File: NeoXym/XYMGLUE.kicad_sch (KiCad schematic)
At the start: 42 parts, among them J1 Conn_01x08, J2 Conn_01x08, SW1 SW_Push, SW2 SW_Push, SW3 SW_SPDT, SW4 SW_SPDT, SW5 SW_Push, U1 74HCT138, U10 74HCT04, U15 74HCT00, U16 74HCT14, U17 74HCT121, U18 NE555P, U2 74HCT138, U4 74HCT32, U5 74HCT00, U6 74HCT09, U8 74HCT10, U9 74HCT00, X1 1.8432MHz

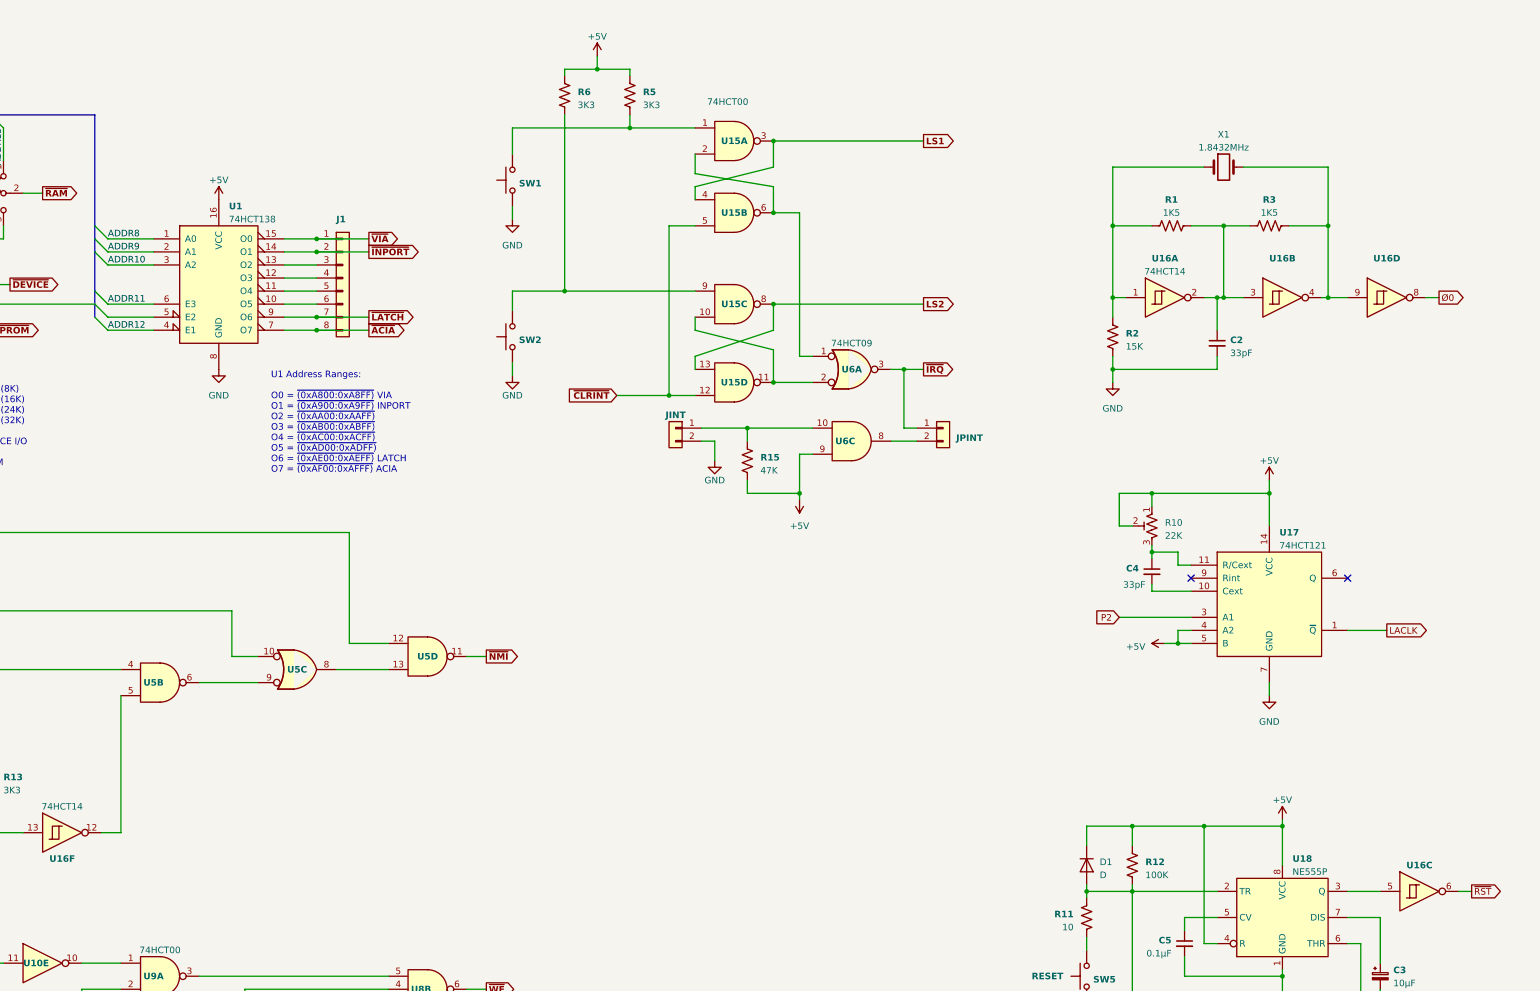
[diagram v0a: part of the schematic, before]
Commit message: modified:   CPU_MEM_IOCTRL.kicad_sch 	modified:   XYMGLUE.kicad_sch 	modified:   XYMPOWER.kicad_sch
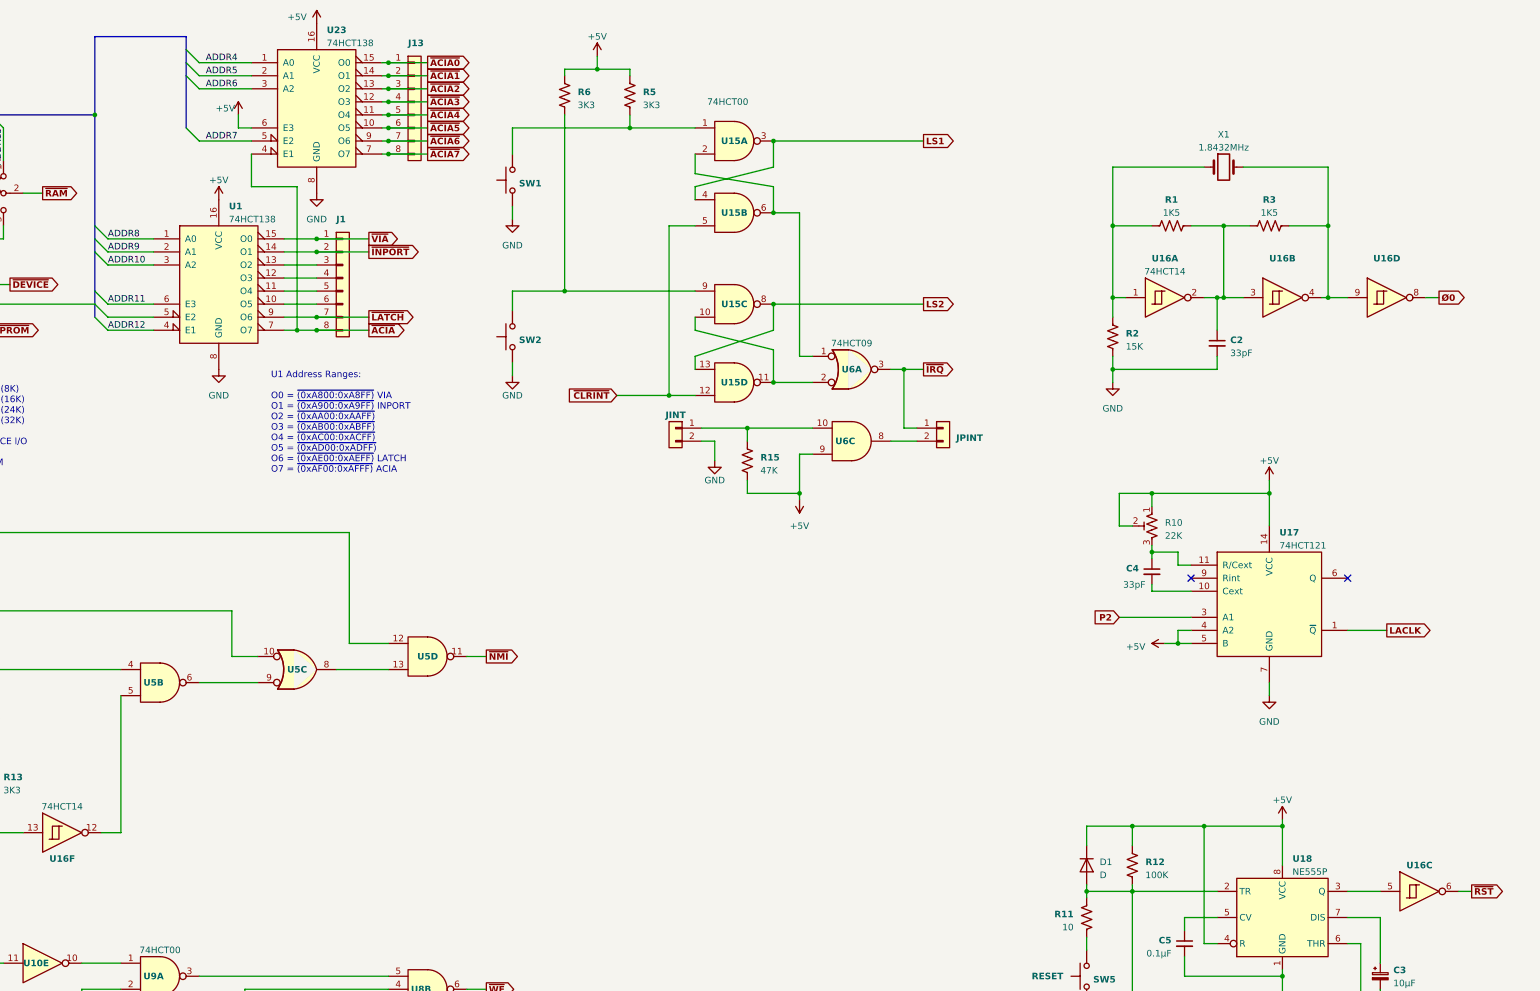
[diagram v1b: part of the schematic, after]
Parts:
- added J13: Conn_01x08, symbol Connector_Generic:Conn_01x08
- added U23: 74HCT138, symbol 74xx:74LS138
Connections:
- net +5V: now also U23.16 (VCC), U23.6 (E3)
- net GND: now also U23.8 (GND)
- net ~{ACIA}: now also U23.4 (E1)
- new net ADDR4: U23.1 (A0)
- new net ADDR5: U23.2 (A1)
- new net ADDR6: U23.3 (A2)
- new net ADDR7: U23.5 (E2)
- new net ~{ACIA0}: J13.1 (Pin_1), U23.15 (O0)
- new net ~{ACIA1}: J13.2 (Pin_2), U23.14 (O1)
- new net ~{ACIA2}: J13.3 (Pin_3), U23.13 (O2)
- new net ~{ACIA3}: J13.4 (Pin_4), U23.12 (O3)
- new net ~{ACIA4}: J13.5 (Pin_5), U23.11 (O4)
- new net ~{ACIA5}: J13.6 (Pin_6), U23.10 (O5)
- new net ~{ACIA6}: J13.7 (Pin_7), U23.9 (O6)
- new net ~{ACIA7}: J13.8 (Pin_8), U23.7 (O7)
